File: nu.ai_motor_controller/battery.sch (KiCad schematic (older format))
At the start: 38 parts, among them J12 XT60_RA_MALE, J13 S4B-XH-A, J14 NP_Screw_Terminal_01x02, J15 XT60_RA_MALE, J16 S4B-XH-A, J17 S4B-XH-A, J18 XT60_RA_FEMALE, Q1 IRF9540N, Q2 SSM3K35AMFV, SW2 TACTILE_SWITCH, SW3 TACTILE_SWITCH

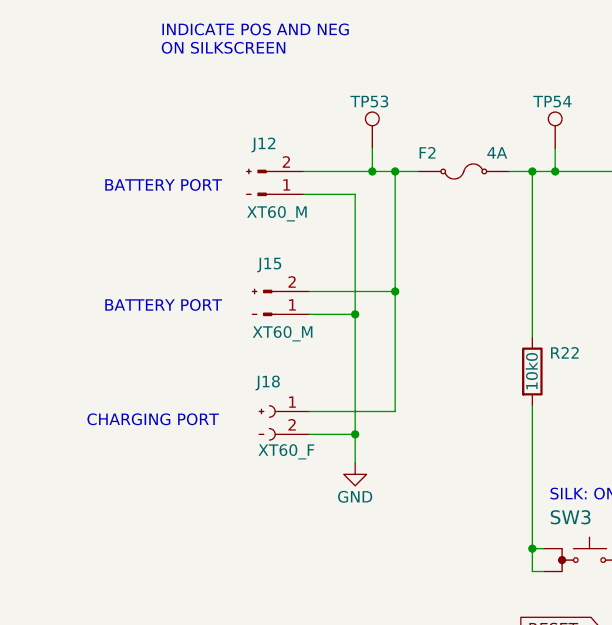
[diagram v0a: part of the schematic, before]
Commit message: automated commit
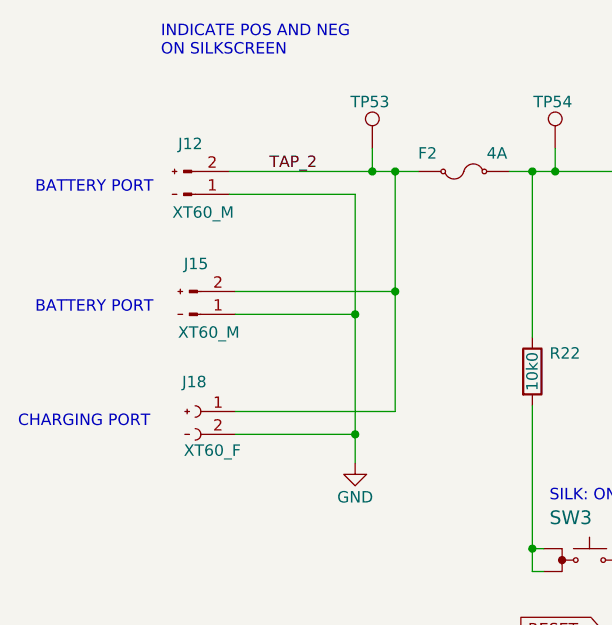
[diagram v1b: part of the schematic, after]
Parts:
- Q1: footprint Package_TO_SOT_THT:TO-220-3_Horizontal_TabDown -> custom:TO-220-3_Horizontal_TabDown
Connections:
- net TAP_2: now also F2.1, J12.2 (Pin_2), J15.2 (Pin_2), J18.1 (Pin_1), TP53.1
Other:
- moved on the sheet: J12, J15, J18
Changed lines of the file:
@@
 	7475 2325 7425 2325
 Wire Wire Line
-	2025 3400 2400 3400
+	1700 3400 2400 3400
 $Comp
 L custom:PTH_0.5_mm TP1
@@
 	2225 3625 2225 3500
 Wire Wire Line
-	2025 3500 2225 3500
+	1700 3500 2225 3500
 $Comp
 L power:GND #PWR057
@@
 	7425 2225 7425 2125
 Wire Wire Line
-	2025 2875 2400 2875
-Wire Wire Line
-	2025 2975 2225 2975
+	1700 2875 2400 2875
+Wire Wire Line
+	1700 2975 2225 2975
 Wire Wire Line
 	2225 2975 2225 3500
@@
 L custom:XT60_RA_MALE J15
 U 1 1 5C51EE4F
-P 1925 2925
-F 0 "J15" H 1800 2725 50  0000 L BNN
-F 1 "XT60_RA_MALE" H 1725 2575 50  0001 L BNN
-F 2 "custom:XT60PW" H 1725 2675 50  0001 L BNN
-F 3 "/home/dj/datasheets/XT60PW.pdf" H 1725 2475 50  0001 L BNN
-F 4 "XT60_M" H 1775 3025 50  0000 L BNN "Text"
-	1    1925 2925
+P 1600 2925
+F 0 "J15" H 1475 2725 50  0000 L BNN
+F 1 "XT60_RA_MALE" H 1400 2575 50  0001 L BNN
+F 2 "custom:XT60PW" H 1400 2675 50  0001 L BNN
+F 3 "/home/dj/datasheets/XT60PW.pdf" H 1400 2475 50  0001 L BNN
+F 4 "XT60_M" H 1450 3025 50  0000 L BNN "Text"
+	1    1600 2925
 	1    0    0    1
 $EndComp
@@
 L custom:XT60_RA_MALE J12
 U 1 1 5C52243D
-P 1900 2400
-F 0 "J12" H 1775 2200 50  0000 L BNN
-F 1 "XT60_RA_MALE" H 1700 2050 50  0001 L BNN
-F 2 "custom:XT60PW" H 1700 2150 50  0001 L BNN
-F 3 "/home/dj/datasheets/XT60PW.pdf" H 1700 1950 50  0001 L BNN
-F 4 "XT60_M" H 1750 2500 50  0000 L BNN "Text"
-	1    1900 2400
+P 1575 2400
+F 0 "J12" H 1450 2200 50  0000 L BNN
+F 1 "XT60_RA_MALE" H 1375 2050 50  0001 L BNN
+F 2 "custom:XT60PW" H 1375 2150 50  0001 L BNN
+F 3 "/home/dj/datasheets/XT60PW.pdf" H 1375 1950 50  0001 L BNN
+F 4 "XT60_M" H 1425 2500 50  0000 L BNN "Text"
+	1    1575 2400
 	1    0    0    1
 $EndComp
@@
 L custom:XT60_RA_FEMALE J18
 U 1 1 5C523072
-P 1950 3450
-F 0 "J18" H 2000 3600 50  0000 L BNN
-F 1 "XT60_RA_FEMALE" H 1750 3100 50  0001 L BNN
-F 2 "custom:XT60PW" H 1750 3200 50  0001 L BNN
-F 3 "/home/dj/datasheets/XT60PW.pdf" H 1750 3000 50  0001 L BNN
-F 4 "XT60_F" H 1850 3300 50  0000 L BNN "Text"
-	1    1950 3450
+P 1625 3450
+F 0 "J18" H 1675 3600 50  0000 L BNN
+F 1 "XT60_RA_FEMALE" H 1425 3100 50  0001 L BNN
+F 2 "custom:XT60PW" H 1425 3200 50  0001 L BNN
+F 3 "/home/dj/datasheets/XT60PW.pdf" H 1425 3000 50  0001 L BNN
+F 4 "XT60_F" H 1525 3300 50  0000 L BNN "Text"
+	1    1625 3450
 	-1   0    0    -1
 $EndComp
@@
 	2225 2975 2225 2450
 Wire Wire Line
-	2225 2450 2000 2450
+	2225 2450 1675 2450
 Connection ~ 2225 2975
 Wire Wire Line
@@
 	1    0    0    1
 $EndComp
-Text Label 9625 3125 0    50   ~ 0
-TAP_2
 Text Label 9625 3325 0    50   ~ 0
 TAP_0
@@
 F 0 "Q1" V 5225 2250 50  0000 L CNN
 F 1 "IRF9540N" V 5150 1975 50  0000 L CNN
-F 2 "Package_TO_SOT_THT:TO-220-3_Horizontal_TabDown" H 5200 2375 50  0001 L CIN
+F 2 "custom:TO-220-3_Horizontal_TabDown" H 5200 2375 50  0001 L CIN
 F 3 "/home/dj/datasheets/irf9540n.pdf" H 5200 2250 50  0001 L BNN
 	1    5000 2450
@@
 Connection ~ 2300 2350
 Wire Wire Line
-	2300 2350 2000 2350
+	2300 2350 1675 2350
 $Comp
 L custom:PTH_0.5_mm TP52
@@
 Wire Wire Line
 	5000 2800 5000 3075
-Text Notes 1125 2450 0    50   ~ 0
+Text Notes 825  2450 0    50   ~ 0
 BATTERY PORT
-Text Notes 1125 2975 0    50   ~ 0
+Text Notes 825  2975 0    50   ~ 0
 BATTERY PORT
-Text Notes 1050 3475 0    50   ~ 0
+Text Notes 750  3475 0    50   ~ 0
 CHARGING PORT
 Text Notes 10200 3350 0    50   ~ 0
@@
 Wire Wire Line
 	9550 4025 9550 4725
+Text Label 9625 3125 0    50   ~ 0
+TAP_2
+Text Label 1850 2350 0    50   ~ 0
+TAP_2
 $EndSCHEMATC
